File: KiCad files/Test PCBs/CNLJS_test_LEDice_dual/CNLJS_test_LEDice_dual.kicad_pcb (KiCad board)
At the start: 2 copper layers, 150 x 150 mm, 112 parts, among them J1 Conn_01x06_Male, J2 Conn_01x14_Male, U1 WS2812-4020_dual, U10 WS2812-4020_dual, U11 WS2812-4020_dual, U12 WS2812-4020_dual, U13 WS2812-4020_dual, U14 WS2812-4020_dual, U15 WS2812-4020_dual, U16 WS2812-4020_dual, U17 WS2812-4020_dual, U18 WS2812-4020_dual, U19 WS2812-4020_dual, U2 WS2812-4020_dual, U20 WS2812-4020_dual, U21 WS2812-4020_dual, U22 WS2812-4020_dual, U23 WS2812-4020_dual, U24 WS2812-4020_dual, U25 WS2812-4020_dual, U26 WS2812-4020_dual, U27 WS2812-4020_dual, U28 WS2812-4020_dual, U29 WS2812-4020_dual, U3 WS2812-4020_dual, U30 WS2812-4020_dual, U31 WS2812-4020_dual, U32 WS2812-4020_dual, U33 WS2812-4020_dual, U34 WS2812-4020_dual, U35 WS2812-4020_dual, U36 WS2812-4020_dual, U37 WS2812-4020_dual, U38 WS2812-4020_dual, U39 WS2812-4020_dual, U4 WS2812-4020_dual, U40 WS2812-4020_dual, U41 WS2812-4020_dual, U42 WS2812-4020_dual, U43 WS2812-4020_dual, U44 WS2812-4020_dual, U45 WS2812-4020_dual, U46 WS2812-4020_dual, U47 WS2812-4020_dual, U48 WS2812-4020_dual, U49 WS2812-4020_dual, U5 WS2812-4020_dual, U50 WS2812-4020_dual, U51 WS2812-4020_dual, U52 WS2812-4020_dual, U53 WS2812-4020_dual, U54 WS2812-4020_dual, U55 WS2812-4020_dual, U56 WS2812-4020_dual, U57 WS2812-4020_dual, U58 WS2812-4020_dual, U59 WS2812-4020_dual, U6 WS2812-4020_dual, U60 WS2812-4020_dual, U61 WS2812-4020_dual, U62 WS2812-4020_dual, U63 WS2812-4020_dual, U64 WS2812-4020_dual, U65 WS2812-4020_dual, U66 WS2812-4020_dual, U67 WS2812-4020_dual, U68 WS2812-4020_dual, U69 WS2812-4020_dual, U7 WS2812-4020_dual, U70 WS2812-4020_dual, U71 WS2812-4020_dual, U72 WS2812-4020_dual, U73 WS2812-4020_dual, U74 WS2812-4020_dual, U75 WS2812-4020_dual, U76 WS2812-4020_dual, U77 WS2812-4020_dual, U78 WS2812-4020_dual, U79 WS2812-4020_dual, U8 WS2812-4020_dual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

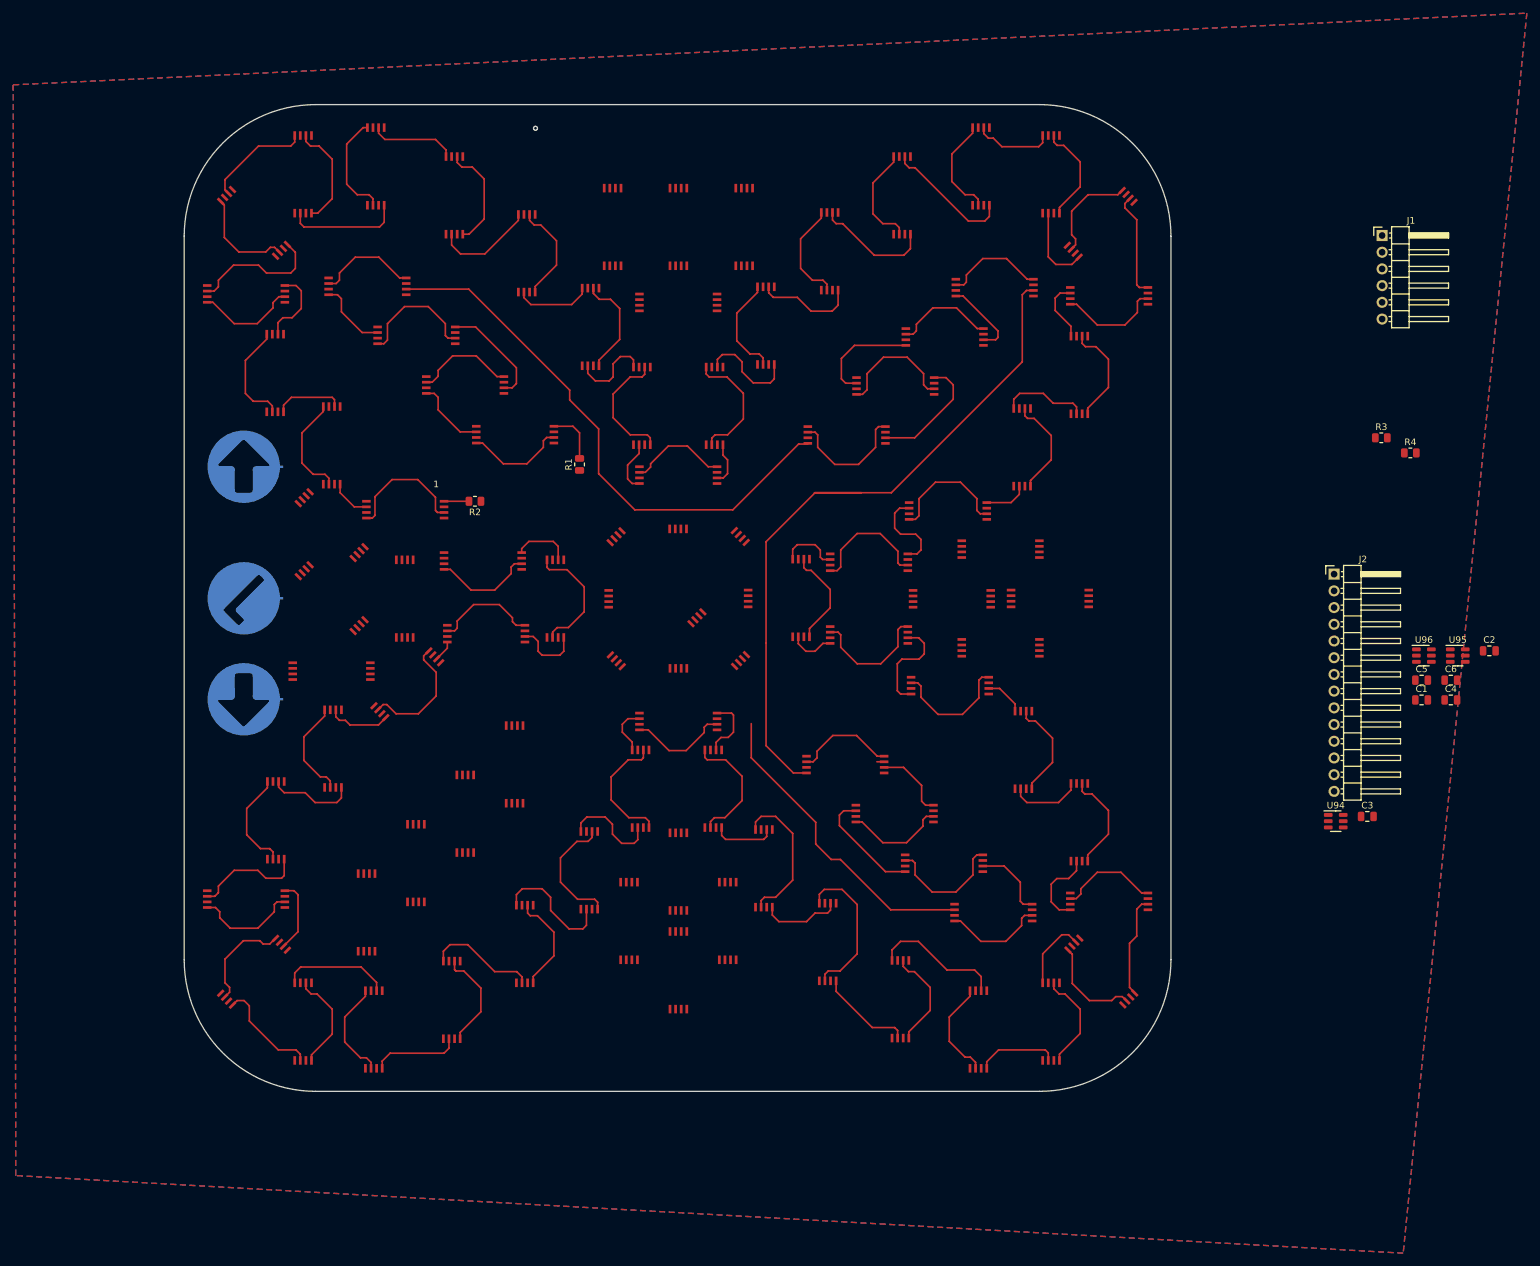
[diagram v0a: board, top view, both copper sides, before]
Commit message: update
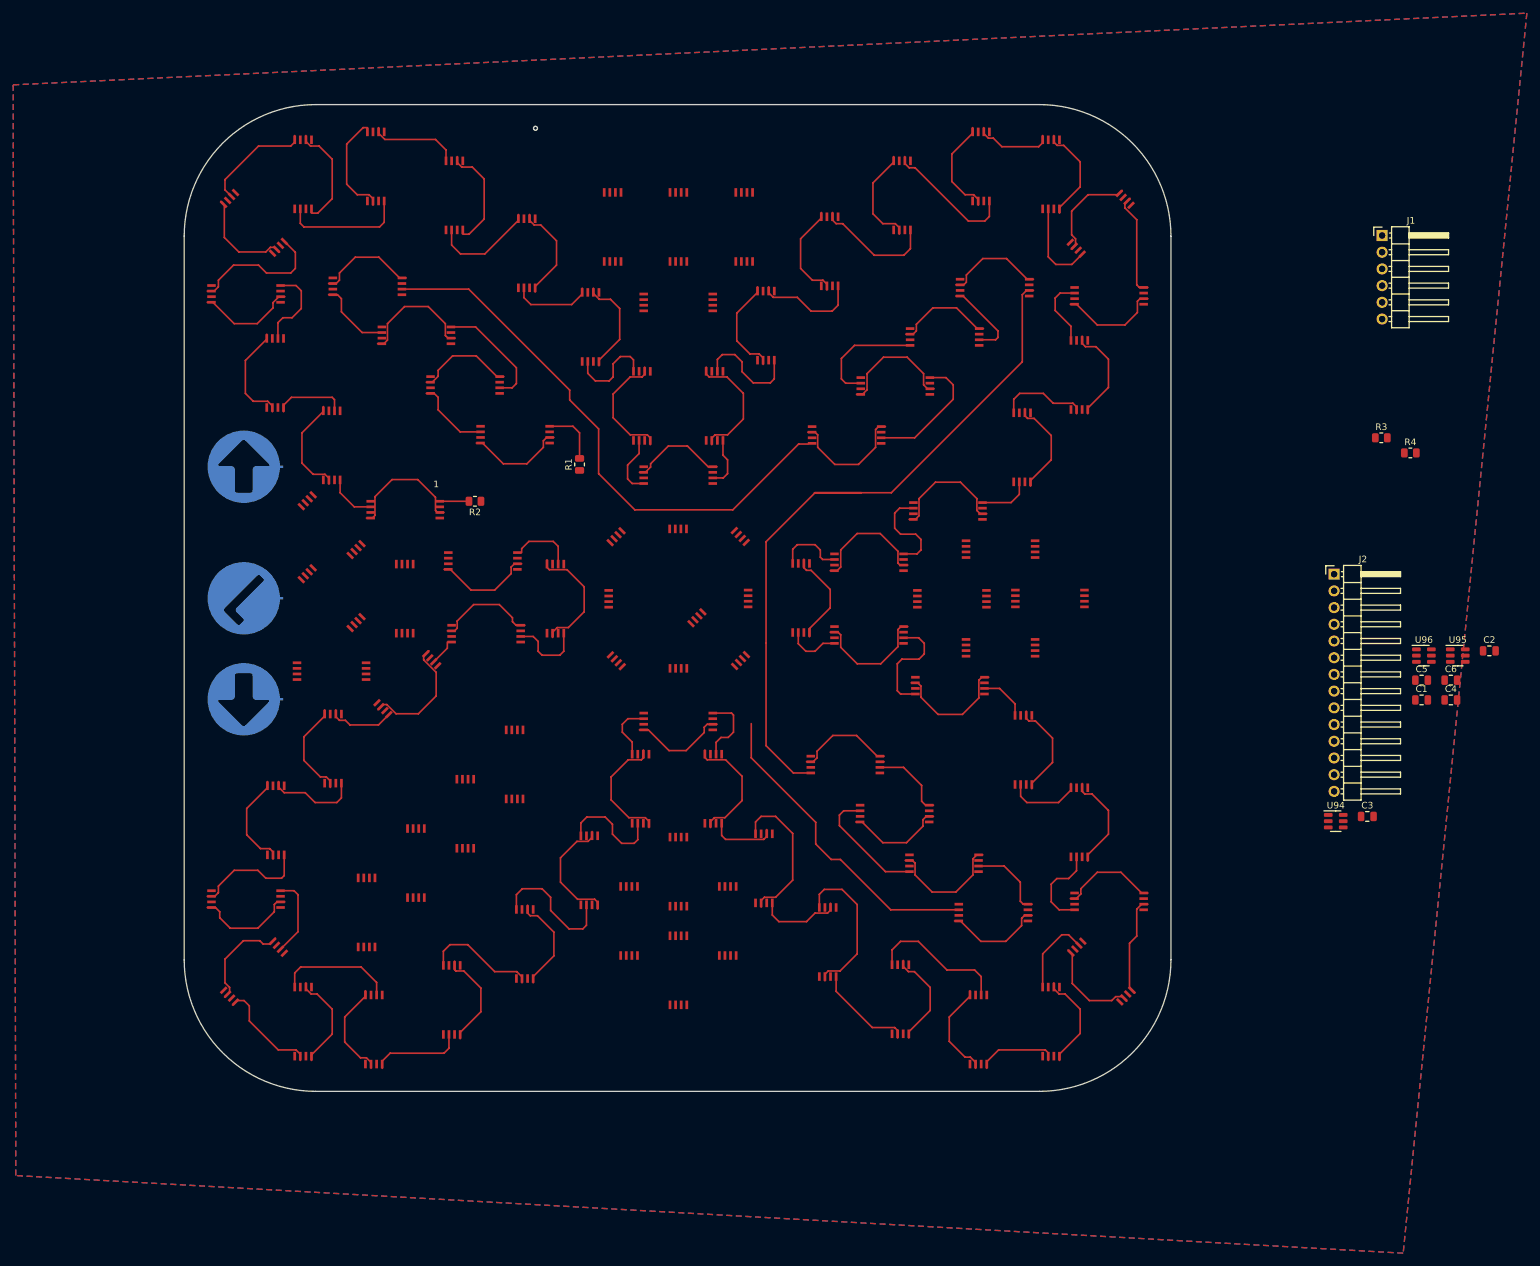
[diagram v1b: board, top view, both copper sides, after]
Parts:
- renumbered U13 to U1, U6 to U10, U7 to U11, U8 to U12, U1 to U13, U2 to U14, U3 to U15, U4 to U16, U14 to U2, U15 to U3, U16 to U4, U9 to U5, U10 to U6, U11 to U7, U12 to U8, U87 to U85, U85 to U87, U90 to U88, U91 to U89, U5 to U9, U92 to U90, U93 to U91, U88 to U92, U89 to U93
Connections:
- U1 pad 1: Net-(U12-Pad5) -> Net-(R1-Pad2)
- U12 pad 5: Net-(U8-Pad5) -> Net-(U12-Pad5)
- U13 pad 1: Net-(R1-Pad2) -> Net-(U12-Pad5)
- U16 pad 5: Net-(U4-Pad5) -> unconnected-(U16-Pad5)
- U4 pad 5: unconnected-(U16-Pad5) -> Net-(U4-Pad5)
- U5 pad 1: Net-(U8-Pad5) -> Net-(U4-Pad5)
- U8 pad 5: Net-(U12-Pad5) -> Net-(U8-Pad5)
- U85 pad 1: Net-(U86-Pad5) -> Net-(R4-Pad2)
- U87 pad 1: Net-(R4-Pad2) -> Net-(U86-Pad4)
- U9 pad 1: Net-(U4-Pad5) -> Net-(U8-Pad5)
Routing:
- net unconnected-(U16-Pad5): track 0.00 -> 84.0 mm
- net Net-(U4-Pad5): track 84.0 -> 0.00 mm
- net Net-(U12-Pad5): track 47.6 -> 116.6 mm
- net Net-(U8-Pad5): track 108.4 -> 47.6 mm
- net (no net): track 1059.0 -> 1024.6 mm
- net VDD: track 1.10 -> 19.8 mm
- net GND: track 0.00 -> 15.8 mm
- net Net-(R1-Pad2): track 8.20 -> 0.00 mm
